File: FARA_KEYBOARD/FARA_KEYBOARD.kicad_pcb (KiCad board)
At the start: 2 copper layers, 93.2 x 39.4 mm, 11 parts, among them J1 Conn_01x07_Pin, SW1 SW_Push, SW2 SW_Push, SW3 SW_Push, SW4 SW_Push, SW5 SW_Push, SW6 SW_Push

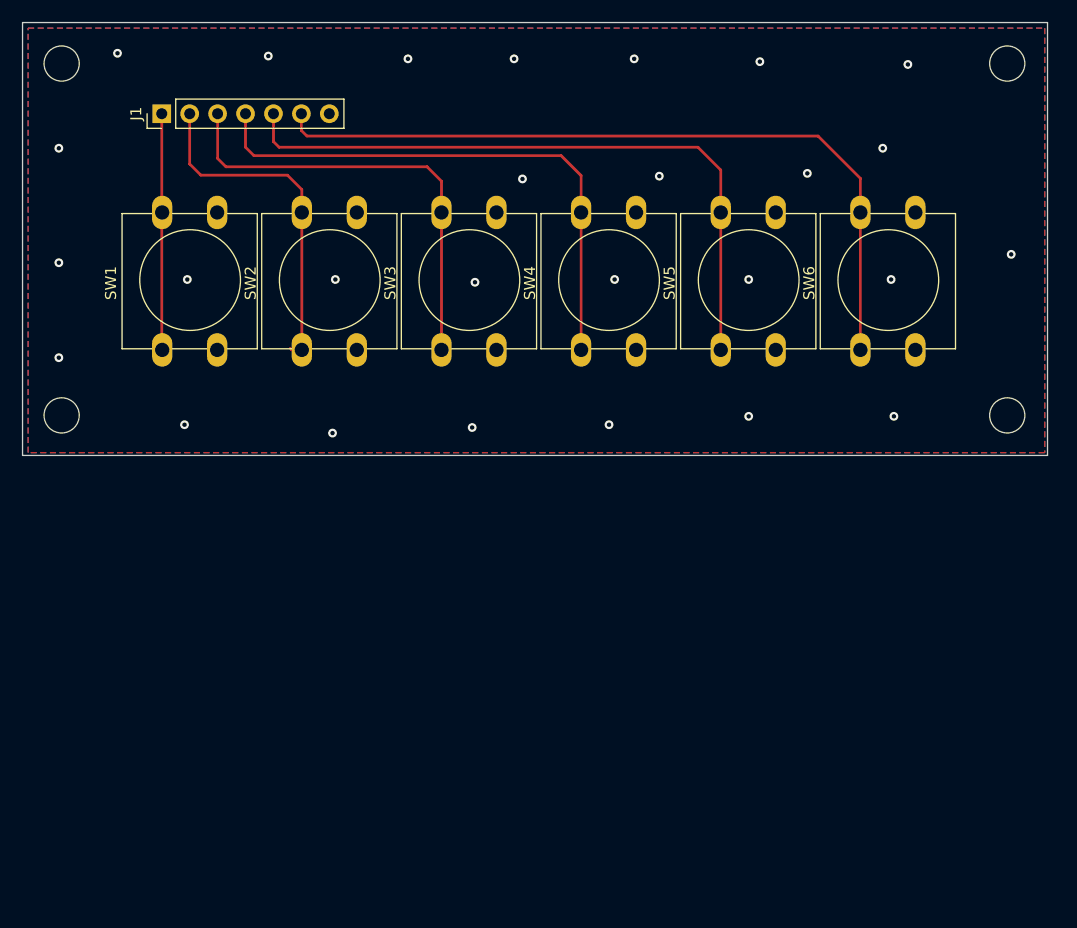
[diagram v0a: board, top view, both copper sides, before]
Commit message: v0.3 Circuit was completed
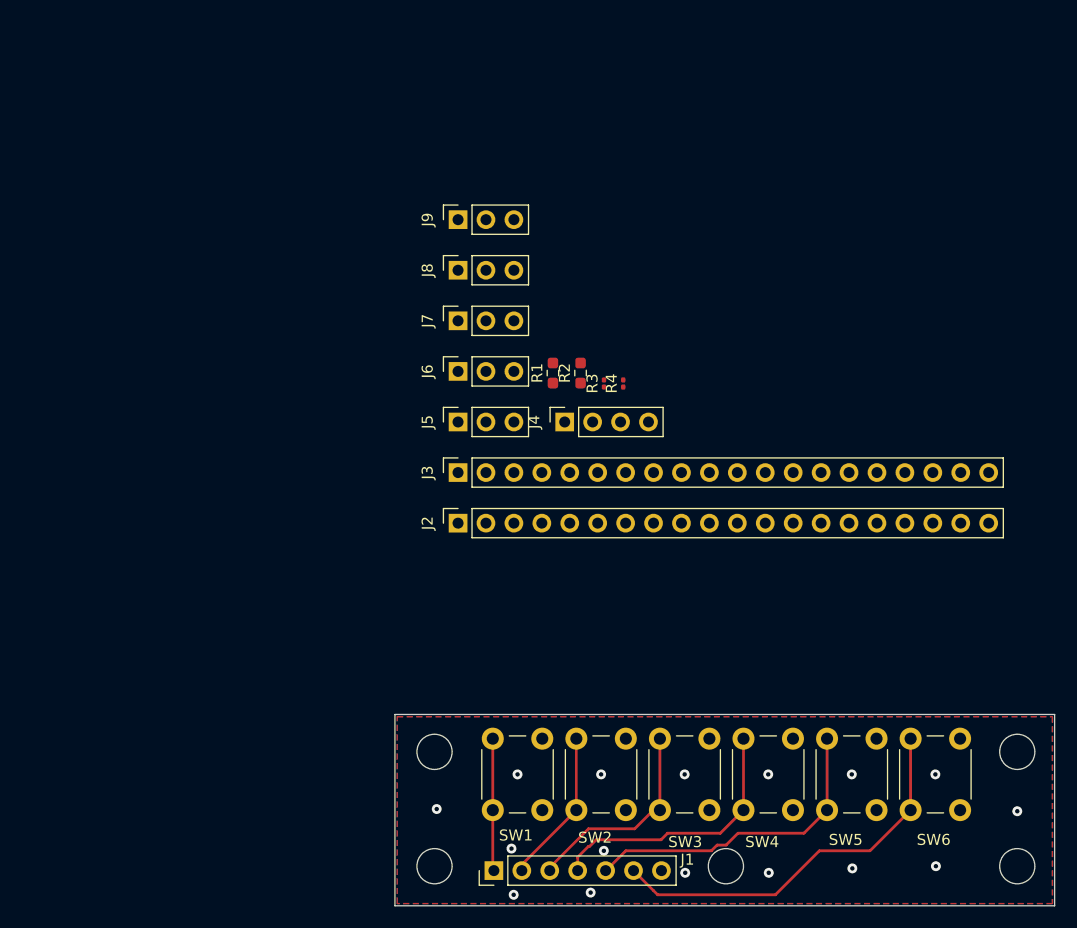
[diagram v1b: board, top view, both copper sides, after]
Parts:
- removed the REF** at (104.3, 53.0)
- removed the REF** at (104.3, 21.0)
- removed the REF** at (18.3, 53.0)
- removed the REF** at (18.3, 21.0)
- added J2: Conn_01x20, Connector_PinSocket_2.54mm:PinSocket_1x20_P2.54mm_Vertical, F.Cu at (54.3, 62.8)
- added J3: Conn_01x20, Connector_PinSocket_2.54mm:PinSocket_1x20_P2.54mm_Vertical, F.Cu at (54.3, 58.2)
- added J4: Conn_01x04, Connector_PinSocket_2.54mm:PinSocket_1x04_P2.54mm_Vertical, F.Cu at (64.0, 53.6)
- added J5: Conn_01x03, Connector_PinSocket_2.54mm:PinSocket_1x03_P2.54mm_Vertical, F.Cu at (54.3, 53.6)
- added J6: Conn_01x03, Connector_PinSocket_2.54mm:PinSocket_1x03_P2.54mm_Vertical, F.Cu at (54.3, 49.0)
- added J7: Conn_01x03, Connector_PinSocket_2.54mm:PinSocket_1x03_P2.54mm_Vertical, F.Cu at (54.3, 44.4)
- added J8: Conn_01x03, Connector_PinSocket_2.54mm:PinSocket_1x03_P2.54mm_Vertical, F.Cu at (54.3, 39.8)
- added J9: Conn_01x03, Connector_PinSocket_2.54mm:PinSocket_1x03_P2.54mm_Vertical, F.Cu at (54.3, 35.2)
- added R1: 4.7k, Resistor_SMD:R_0603_1608Metric_Pad0.98x0.95mm_HandSolder, F.Cu at (63.0, 49.1)
- added R2: 4.7k, Resistor_SMD:R_0603_1608Metric_Pad0.98x0.95mm_HandSolder, F.Cu at (65.5, 49.1)
- added R3: 0, Resistor_SMD:R_0201_0603Metric, F.Cu at (67.6, 50.1)
- added R4: 0, Resistor_SMD:R_0201_0603Metric, F.Cu at (69.4, 50.1)
- added REF**: MountingHole_3.2mm_M3, MountingHole:MountingHole_3.2mm_M3, F.Cu at (105.2, 94.0)
- added REF**: MountingHole_3.2mm_M3, MountingHole:MountingHole_3.2mm_M3, F.Cu at (105.2, 83.6)
- added REF**: MountingHole_3.2mm_M3, MountingHole:MountingHole_3.2mm_M3, F.Cu at (52.2, 94.0)
- added REF**: MountingHole_3.2mm_M3, MountingHole:MountingHole_3.2mm_M3, F.Cu at (52.2, 83.6)
- added REF**: MountingHole_3.2mm_M3, MountingHole:MountingHole_3.2mm_M3, F.Cu at (78.7, 94.0)
- SW1, SW2, SW3, SW4, SW5, SW6: footprint Button_Switch_THT:SW_PUSH-12mm -> Button_Switch_THT:SW_PUSH_6mm
- moved J1 75.2 mm to (57.6, 94.4)
- moved SW1 51.5 mm to (57.5, 88.9)
- moved SW2 48.7 mm to (65.1, 88.9)
- moved SW3 46.3 mm to (72.7, 88.9)
- moved SW4 44.4 mm to (80.3, 88.9)
- moved SW5 43.0 mm to (87.9, 88.9)
- moved SW6 42.1 mm to (95.5, 88.9)
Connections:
- net Net-(J1-Pin_1) renamed SW1
- net Net-(J1-Pin_2) renamed SW2
- net Net-(J1-Pin_3) renamed SW3
- net Net-(J1-Pin_4) renamed SW4
- net Net-(J1-Pin_5) renamed SW5
- net Net-(J1-Pin_6) renamed SW6
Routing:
- net SW6: track 69.8 -> 35.8 mm
- net SW5: track 60.6 -> 28.9 mm
- net SW4: track 50.5 -> 24.6 mm
- net SW3: track 40.6 -> 19.0 mm
- net SW2: track 31.4 -> 14.1 mm
- net SW1: track 21.5 -> 12.7 mm
- net GND: vias 27 -> 16
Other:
- board size 93.2 x 39.4 mm -> 60 x 17.4 mm
